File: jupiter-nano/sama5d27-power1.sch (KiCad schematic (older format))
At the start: 50 parts, among them U1 ATSAMA5D27C-LD1G-CU

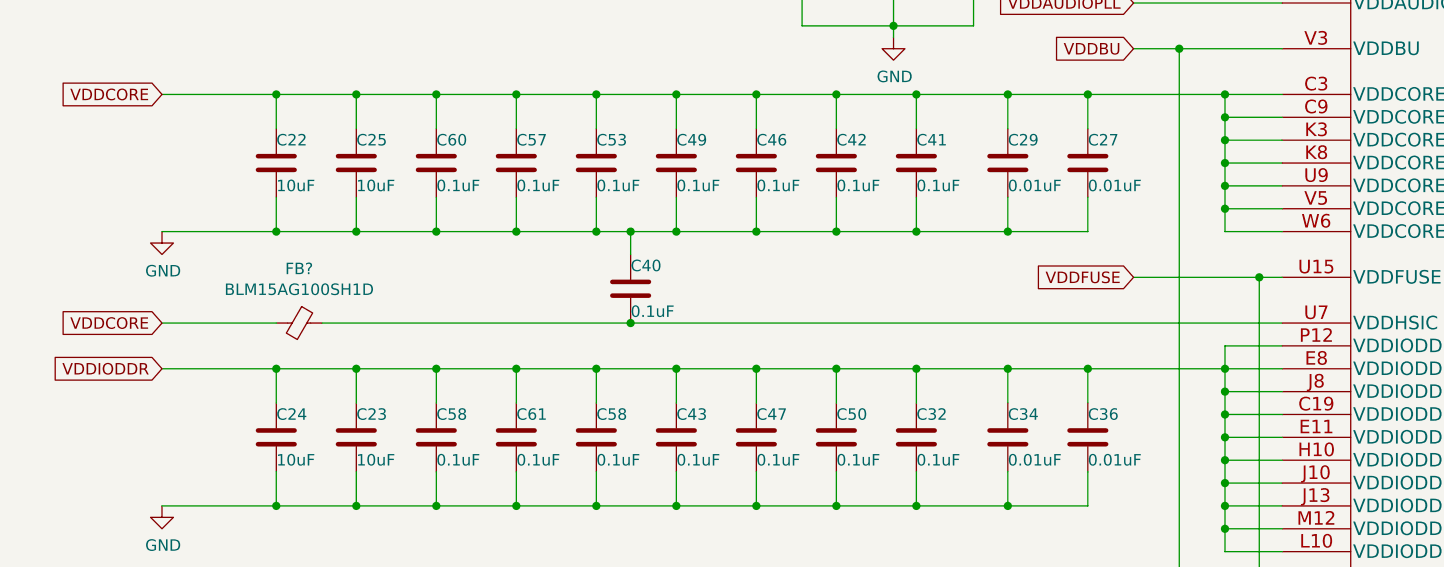
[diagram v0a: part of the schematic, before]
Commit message: cleanup
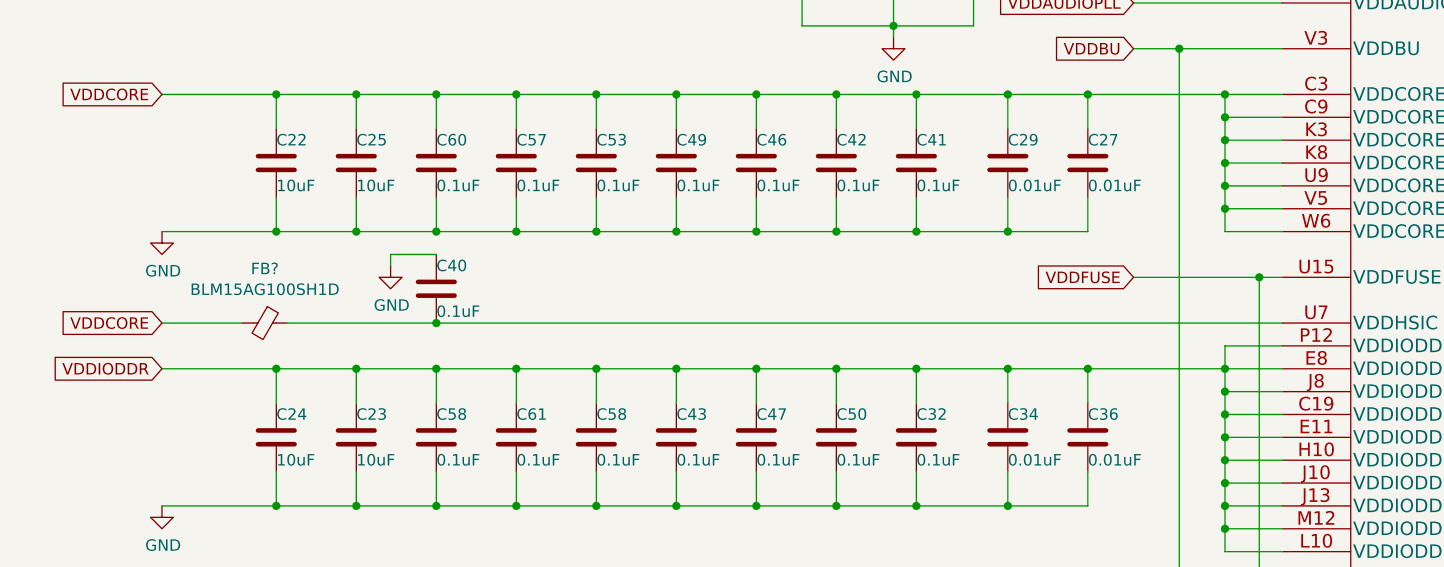
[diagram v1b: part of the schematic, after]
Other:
- moved on the sheet: C40, FB?
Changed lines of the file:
@@
 L Device:Ferrite_Bead_Small FB?
 U 1 1 5F91D238
-P 4500 3450
+P 4350 3450
 AR Path="/5F395E67/5F91D238" Ref="FB?"  Part="1"
 AR Path="/5FD740BF/5F91D238" Ref="FB?"  Part="1"
-F 0 "FB?" V 4263 3450 50  0000 C CNN
-F 1 "BLM15AG100SH1D" V 4354 3450 50  0000 C CNN
-F 2 "Capacitor_SMD:C_0402_1005Metric" V 4430 3450 50  0001 C CNN
-F 3 "~" H 4500 3450 50  0001 C CNN
-	1    4500 3450
+F 0 "FB?" V 4113 3450 50  0000 C CNN
+F 1 "BLM15AG100SH1D" V 4204 3450 50  0000 C CNN
+F 2 "Capacitor_SMD:C_0402_1005Metric" V 4280 3450 50  0001 C CNN
+F 3 "~" H 4350 3450 50  0001 C CNN
+	1    4350 3450
 	0    1    1    0
 $EndComp
 Wire Wire Line
-	4400 3450 3900 3450
+	4250 3450 3900 3450
 Wire Wire Line
-	4600 3450 5950 3450
-Connection ~ 5950 3450
-Wire Wire Line
-	5950 3450 8800 3450
-Wire Wire Line
-	5800 3050 5950 3050
-Connection ~ 5950 3050
-Wire Wire Line
-	5950 3050 6150 3050
-Wire Wire Line
-	5950 3150 5950 3050
+	4450 3450 5100 3450
 $Comp
 L Device:C C40
 U 1 1 5F9EE154
-P 5950 3300
-F 0 "C40" H 5950 3400 50  0000 L CNN
-F 1 "0.1uF" H 5950 3200 50  0000 L CNN
-F 2 "" H 5988 3150 50  0001 C CNN
-F 3 "~" H 5950 3300 50  0001 C CNN
-	1    5950 3300
+P 5100 3300
+F 0 "C40" H 5100 3400 50  0000 L CNN
+F 1 "0.1uF" H 5100 3200 50  0000 L CNN
+F 2 "" H 5138 3150 50  0001 C CNN
+F 3 "~" H 5100 3300 50  0001 C CNN
+	1    5100 3300
 	1    0    0    -1
 $EndComp
@@
 Text GLabel 7950 700  0    50   Input ~ 0
 VDD_3V3
+Connection ~ 5100 3450
+Wire Wire Line
+	5800 3050 6150 3050
+Wire Wire Line
+	5100 3450 8800 3450
+Wire Wire Line
+	5100 3150 4900 3150
+Wire Wire Line
+	4900 3150 4900 3200
+$Comp
+L power:GND #PWR?
+U 1 1 602286E4
+P 4900 3200
+F 0 "#PWR?" H 4900 2950 50  0001 C CNN
+F 1 "GND" H 4905 3027 50  0000 C CNN
+F 2 "" H 4900 3200 50  0001 C CNN
+F 3 "" H 4900 3200 50  0001 C CNN
+	1    4900 3200
+	1    0    0    -1
+$EndComp
 $EndSCHEMATC
